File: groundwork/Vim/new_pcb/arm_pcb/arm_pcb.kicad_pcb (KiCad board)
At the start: 2 copper layers, 81.3 x 61 mm, 22 parts, among them U1 NODEMCU32S

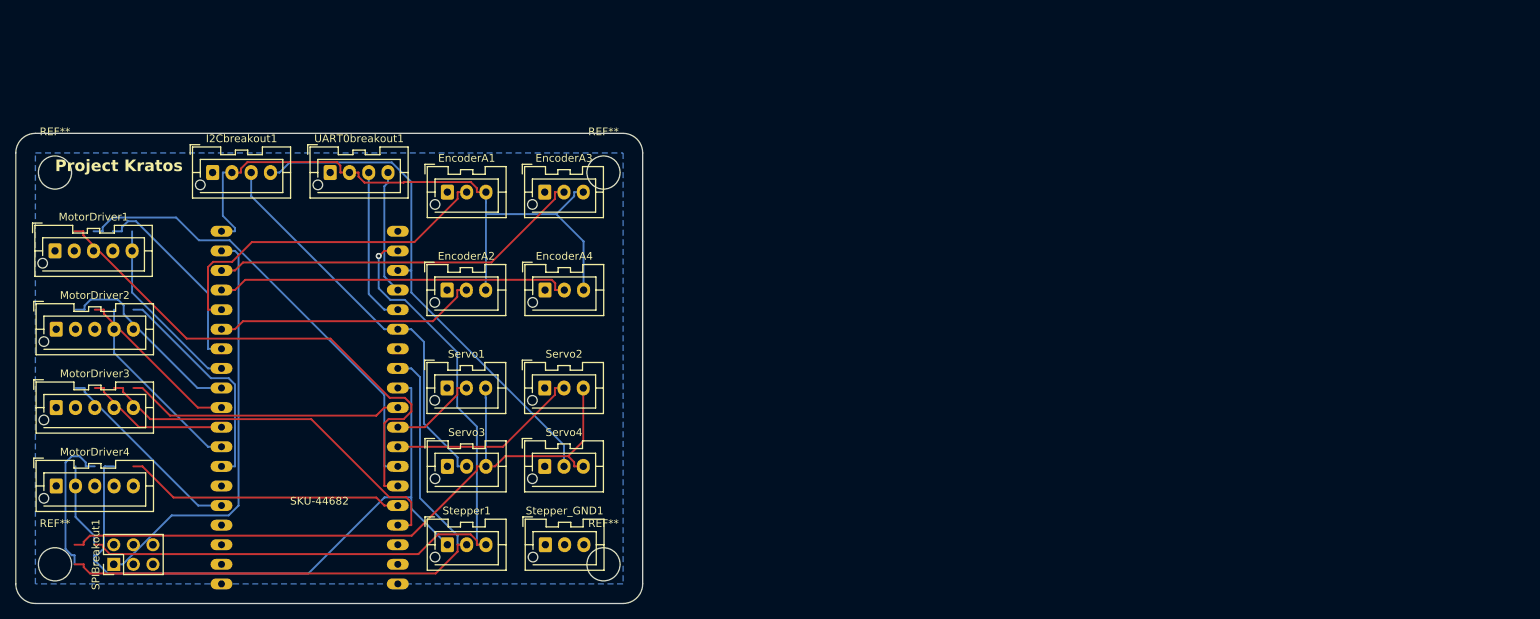
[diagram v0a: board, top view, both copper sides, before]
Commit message: final pcb v0.2
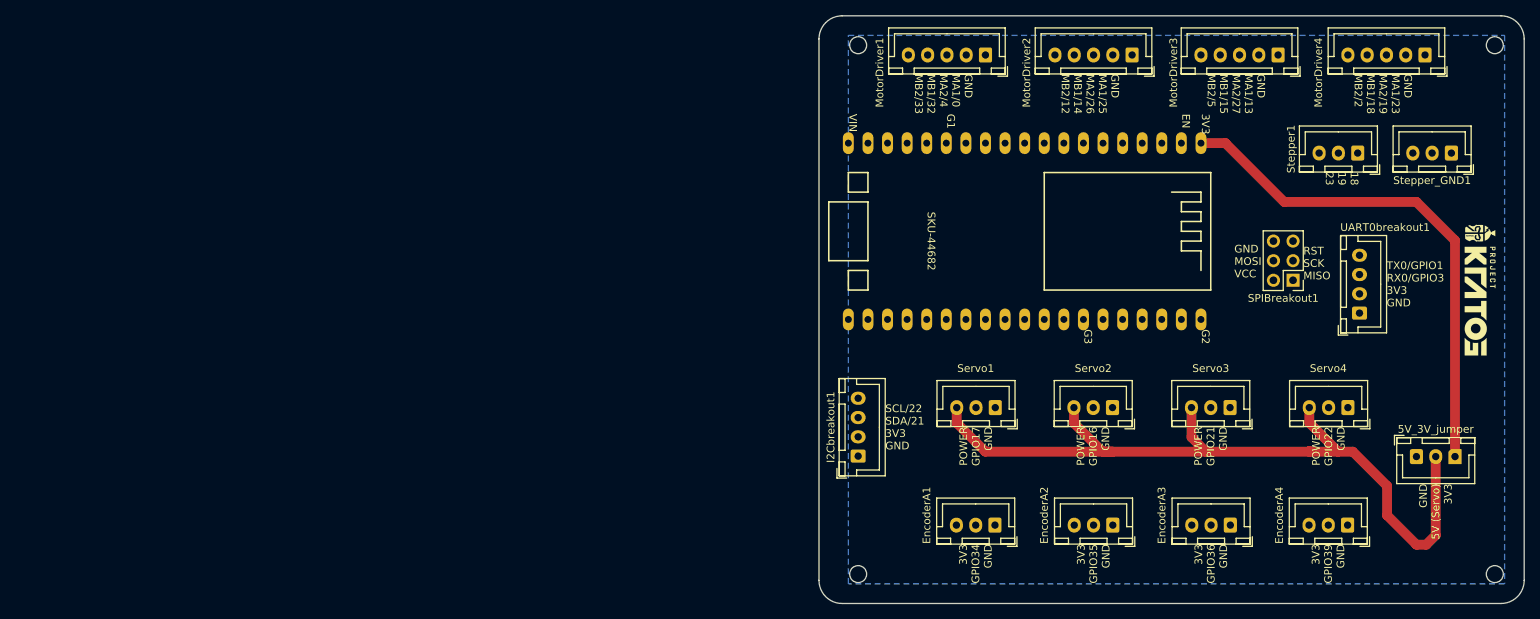
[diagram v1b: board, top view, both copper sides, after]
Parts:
- removed REF** (x4): MountingHole_4.3mm_M4, MountingHole:MountingHole_4.3mm_M4
- added 5V_3V_jumper: JST_XH_B3B-XH-A_1x03_P2.50mm_Vertical, Connector_JST:JST_XH_B3B-XH-A_1x03_P2.50mm_Vertical, F.Cu at (229.9, 108.0)
- added G***: LOGO, LOGO, F.Cu at (238.1, 86.4)
- added mountinghole1: MountingHole_2.2mm_M2, MountingHole:MountingHole_2.2mm_M2, F.Cu at (157.5, 54.6)
- added mountinghole2: MountingHole_2.2mm_M2, MountingHole:MountingHole_2.2mm_M2, F.Cu at (157.5, 123.2)
- added mountinghole3: MountingHole_2.2mm_M2, MountingHole:MountingHole_2.2mm_M2, F.Cu at (240.0, 123.2)
- added mountinghole4: MountingHole_2.2mm_M2, MountingHole:MountingHole_2.2mm_M2, F.Cu at (240.0, 54.6)
- EncoderA1, EncoderA2, EncoderA3, EncoderA4, Servo1, Servo2, Servo3, Servo4, Stepper1, Stepper_GND1: footprint Connector_JST:JST_XA_B03B-XASK-1-A_1x03_P2.50mm_Vertical -> Connector_JST:JST_XH_B3B-XH-A_1x03_P2.50mm_Vertical
- I2Cbreakout1, UART0breakout1: footprint Connector_JST:JST_XA_B04B-XASK-1-A_1x04_P2.50mm_Vertical -> Connector_JST:JST_XH_B4B-XH-A_1x04_P2.50mm_Vertical
- MotorDriver1, MotorDriver2, MotorDriver3, MotorDriver4: footprint Connector_JST:JST_XA_B05B-XASK-1-A_1x05_P2.50mm_Vertical -> Connector_JST:JST_XH_B5B-XH-A_1x05_P2.50mm_Vertical
- moved MotorDriver4 186.1 mm to (231.0, 55.9), turned to 180 degrees
- moved MotorDriver3 164.9 mm to (211.9, 55.9), turned to 180 degrees
- moved SPIBreakout1 157.3 mm to (213.9, 85.1), turned to 180 degrees
- moved MotorDriver2 144.0 mm to (193.0, 55.9), turned to 180 degrees
- moved UART0breakout1 134.7 mm to (222.5, 89.3), turned to 90 degrees
- moved Stepper1 128.5 mm to (222.2, 68.6), turned to 180 degrees
- moved Stepper_GND1 128.0 mm to (234.4, 68.6), turned to 180 degrees
- moved MotorDriver1 123.3 mm to (174.0, 55.9), turned to 180 degrees
- moved EncoderA4 108.4 mm to (220.9, 116.8), turned to 180 degrees
- moved Servo4 104.4 mm to (221.0, 101.6), turned to 180 degrees
- moved Servo3 101.8 mm to (205.7, 101.6), turned to 180 degrees
- moved EncoderA3 98.8 mm to (205.7, 116.8), turned to 180 degrees
- moved U1 96.4 mm to (180.3, 78.7), turned to -90 degrees
- moved EncoderA2 91.5 mm to (190.5, 116.8), turned to 180 degrees
- moved I2Cbreakout1 91.4 mm to (157.5, 107.9), turned to 90 degrees
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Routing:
- net SPI_MOSI: track 112.4 -> 0.00 mm, vias 1 -> 0
- net SPI_MISO: track 100.8 -> 0.00 mm
- net SPI_SCK: track 84.6 -> 0.00 mm
- net m1_1: track 68.3 -> 0.00 mm
- net servo4: track 66.7 -> 0.00 mm
- net m1_2: track 59.3 -> 0.00 mm
- net SPI_RST: track 54.3 -> 0.00 mm
- net servo3: track 52.4 -> 0.00 mm
- net Net-(MotorDriver3-Pin_4): track 49.7 -> 0.00 mm
- net a_in_3: track 49.1 -> 0.00 mm
- net a_in_4: track 46.1 -> 0.00 mm
- net a_in_1: track 45.4 -> 0.00 mm
- net m4_4: track 36.4 -> 0.00 mm
- net Net-(MotorDriver3-Pin_5): track 36.2 -> 0.00 mm
- net a_in_2: track 34.4 -> 0.00 mm
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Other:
- board size 81.3 x 61 mm -> 91.4 x 76.2 mm
- board text added: "18 19 23"
- board text added: "3V3 GPIO34 GND"
- board text added: "3V3 GPIO35 GND"
- board text added: "3V3 GPIO36 GND"
- board text added: "3V3 GPIO39 GND"
- board text added: "GND 5V (Servo) 3V3"
- board text added: "GND MA1/0 MA2/4 MB1/32 MB2/33"
- board text added: "GND MA1/13 MA2/27 MB1/15 MB2/5"
- board text added: "GND MA1/23 MA2/19 MB1/18 MB2/2"
- board text added: "GND MA1/25 MA2/26 MB1/14 MB2/12"
- board text added: "GND MOSI VCC"
- board text added: "POWER GPIO16 GND"
- board text added: "POWER GPIO17 GND"
- board text added: "POWER GPIO21 GND"
- board text added: "POWER GPIO22 GND"
- board text added: "RST SCK MISO"
- board text added: "SCL/22 SDA/21 3V3 GND"
- board text added: "TX0/GPIO1 RX0/GPIO3 3V3 GND"
- board text removed: "Project Kratos"
